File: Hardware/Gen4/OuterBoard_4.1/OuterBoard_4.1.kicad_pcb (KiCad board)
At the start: 6 copper layers, 47.9 x 31.8 mm, 104 parts, among them J1 6130XX11121_61300611121, J10 F32R-1A7H1-11024, J2 6130XX11121_61300611121, J3 530470210, J4 530470210, J6 10118194-0001LF, SW1 PTS815 SJM 250 SMTR LFS, SW3 PTS815 SJM 250 SMTR LFS, U1 MCP73812T-420I-OT, U2 GD25Q64CSIGR, U3 MCP73812T-420I-OT, U4 AZ1117CH-3.3TRG1, U5 MIC5504-1.8YM5, U7 TLV75528PDBVR, U8 BNO055, U9 ESP32-S3, Y1 ABS07-32.768KHZ-7-T, Y2 ABM8G-40.000MHZ-18-D2Y-T

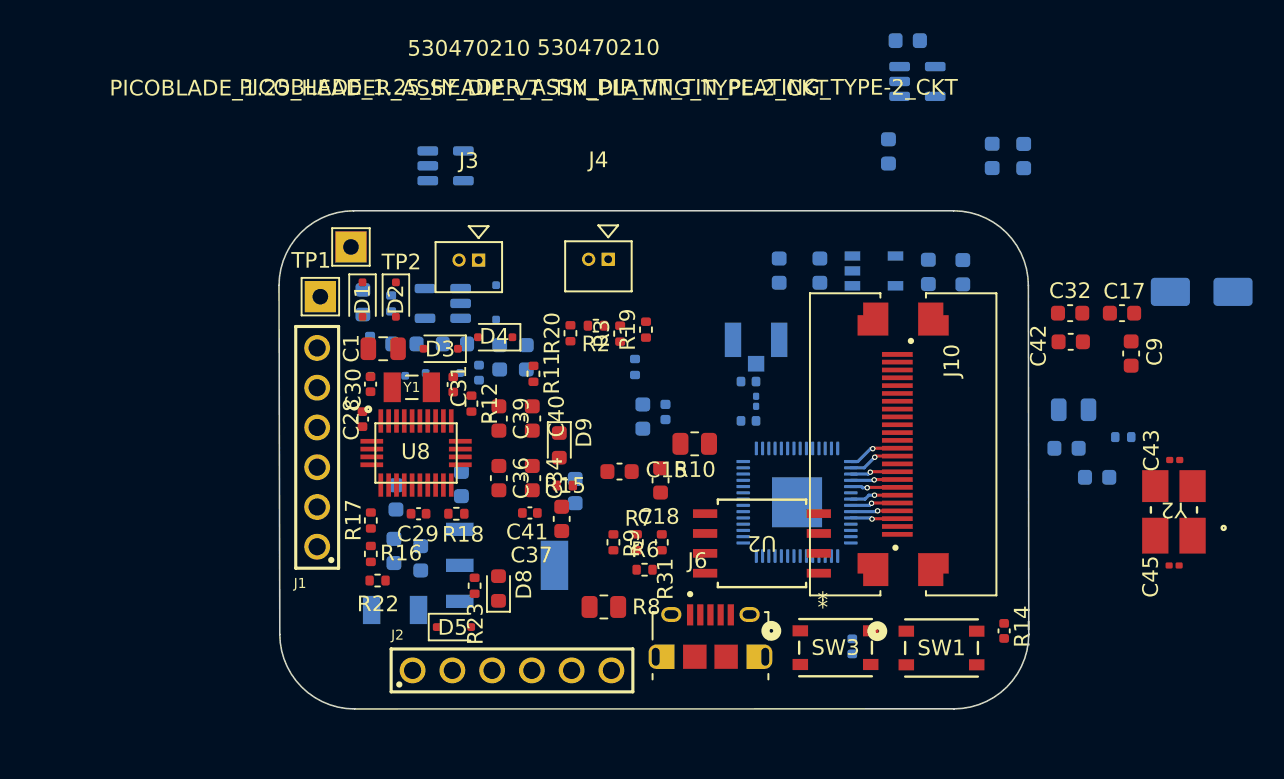
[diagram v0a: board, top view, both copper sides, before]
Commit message: stuff
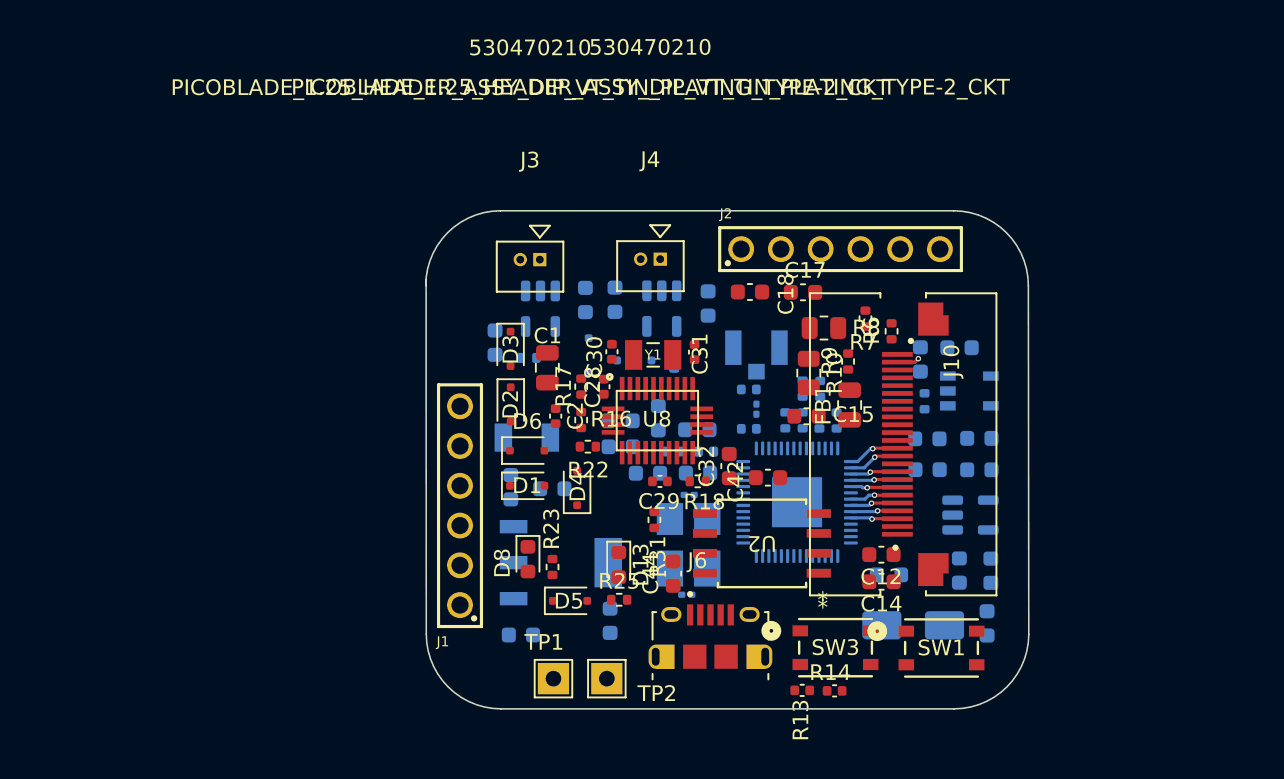
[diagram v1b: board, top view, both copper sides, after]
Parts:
- C12, C14, C2, C44, D13, D6, FB1, R13, R25: moved to F.Cu
- C34, C36, C37, C39, C40, C41, C43, C45, C9, D9, R11, R12, R15, R19, R2, R20, R3, Y2: moved to B.Cu
- moved J2 34.1 mm to (143.0, 77.1)
- moved TP2 32.1 mm to (128.0, 104.5)
- moved C45 31.2 mm to (133.1, 99.2), turned to 0 degrees
- moved C43 31.1 mm to (133.3, 92.8), turned to 180 degrees
- moved Y2 31.1 mm to (133.3, 95.9), turned to 0 degrees
- moved TP1 28.6 mm to (124.6, 104.5)
- moved D7 28.2 mm to (147.6, 101.1), turned to 0 degrees
- moved U5 27.9 mm to (151.3, 94.1)
- moved C21 27.4 mm to (148.5, 91.2), turned to 180 degrees
- moved C24 26.6 mm to (150.6, 97.6)
- moved C26 26.6 mm to (152.6, 97.6)
- moved R15 24.0 mm to (148.7, 97.8)
- moved C32 23.9 mm to (135.8, 91.0), turned to 90 degrees
- moved D13 23.4 mm to (128.8, 97.3)
- moved R25 22.8 mm to (128.8, 99.5), turned to 0 degrees
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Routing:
- net GND: track 0.00 -> 1.43 mm, vias 0 -> 1
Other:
- board size 47.9 x 31.8 mm -> 38.5 x 31.8 mm
